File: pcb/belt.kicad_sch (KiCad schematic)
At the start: 10 parts, among them SW1 RESET, U1 Raspberry-Pi-Pico

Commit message: modified footprints
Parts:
- D1, D2: footprint (none) -> LED_THT:LED_D5.0mm
- H1, H2, H3, H4: footprint (none) -> MountingHole:MountingHole_2.7mm_M2.5
- R1, R2: footprint (none) -> Resistor_THT:R_Axial_DIN0207_L6.3mm_D2.5mm_P10.16mm_Horizontal
- SW1: footprint (none) -> Button_Switch_THT:SW_PUSH_6mm_H5mm
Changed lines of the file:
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@@
       (effects (font (size 1.27 1.27)) (justify left))
     )
-    (property "Footprint" "" (at 253.492 81.28 90)
+    (property "Footprint" "Resistor_THT:R_Axial_DIN0207_L6.3mm_D2.5mm_P10.16mm_Horizontal" (at 253.492 81.28 90)
       (effects (font (size 1.27 1.27)) hide)
     )
@@
       (effects (font (size 1.27 1.27)) (justify left))
     )
-    (property "Footprint" "" (at 234.95 114.3 0)
+    (property "Footprint" "MountingHole:MountingHole_2.7mm_M2.5" (at 234.95 114.3 0)
       (effects (font (size 1.27 1.27)) hide)
     )
@@
       (effects (font (size 1.27 1.27)) (justify right))
     )
-    (property "Footprint" "" (at 255.27 71.12 0)
+    (property "Footprint" "LED_THT:LED_D5.0mm" (at 255.27 71.12 0)
       (effects (font (size 1.27 1.27)) hide)
     )
@@
       (effects (font (size 1.27 1.27)))
     )
-    (property "Footprint" "" (at 44.45 58.42 0)
+    (property "Footprint" "Button_Switch_THT:SW_PUSH_6mm_H5mm" (at 44.45 58.42 0)
       (effects (font (size 1.27 1.27)) hide)
     )
@@
       (effects (font (size 1.27 1.27)) (justify left))
     )
-    (property "Footprint" "" (at 234.95 127 0)
+    (property "Footprint" "MountingHole:MountingHole_2.7mm_M2.5" (at 234.95 127 0)
       (effects (font (size 1.27 1.27)) hide)
     )
@@
       (effects (font (size 1.27 1.27)) (justify left))
     )
-    (property "Footprint" "" (at 234.95 133.35 0)
+    (property "Footprint" "MountingHole:MountingHole_2.7mm_M2.5" (at 234.95 133.35 0)
       (effects (font (size 1.27 1.27)) hide)
     )
@@
       (effects (font (size 1.27 1.27)) (justify left))
     )
-    (property "Footprint" "" (at 235.712 81.28 90)
+    (property "Footprint" "Resistor_THT:R_Axial_DIN0207_L6.3mm_D2.5mm_P10.16mm_Horizontal" (at 235.712 81.28 90)
       (effects (font (size 1.27 1.27)) hide)
     )
@@
       (effects (font (size 1.27 1.27)) (justify left))
     )
-    (property "Footprint" "" (at 234.95 120.65 0)
+    (property "Footprint" "MountingHole:MountingHole_2.7mm_M2.5" (at 234.95 120.65 0)
       (effects (font (size 1.27 1.27)) hide)
     )
@@
       (effects (font (size 1.27 1.27)) (justify right))
     )
-    (property "Footprint" "" (at 237.49 71.12 0)
-      (effects (font (size 1.27 1.27)) hide)
-    )
+    (property "Footprint" "LED_THT:LED_D5.0mm" (at 237.49 71.12 0)
+      (effects (font (size 1.27 1.27)) hide)
+    )

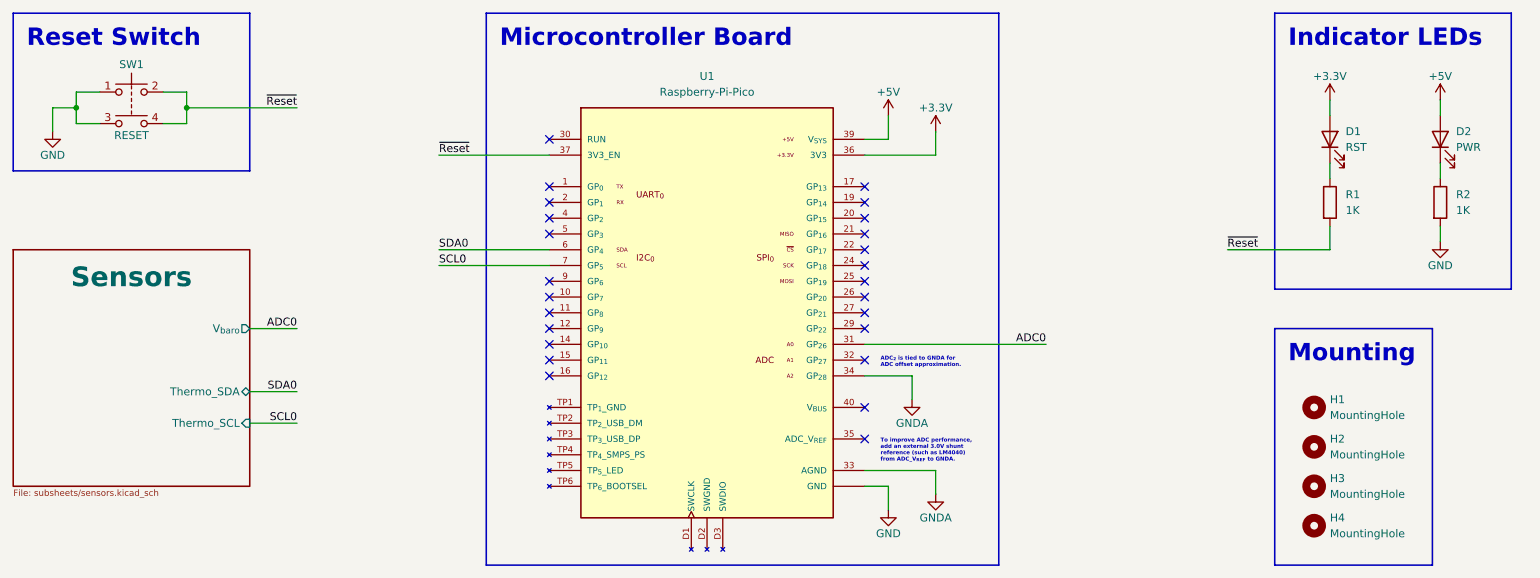
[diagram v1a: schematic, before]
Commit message: ready for layout
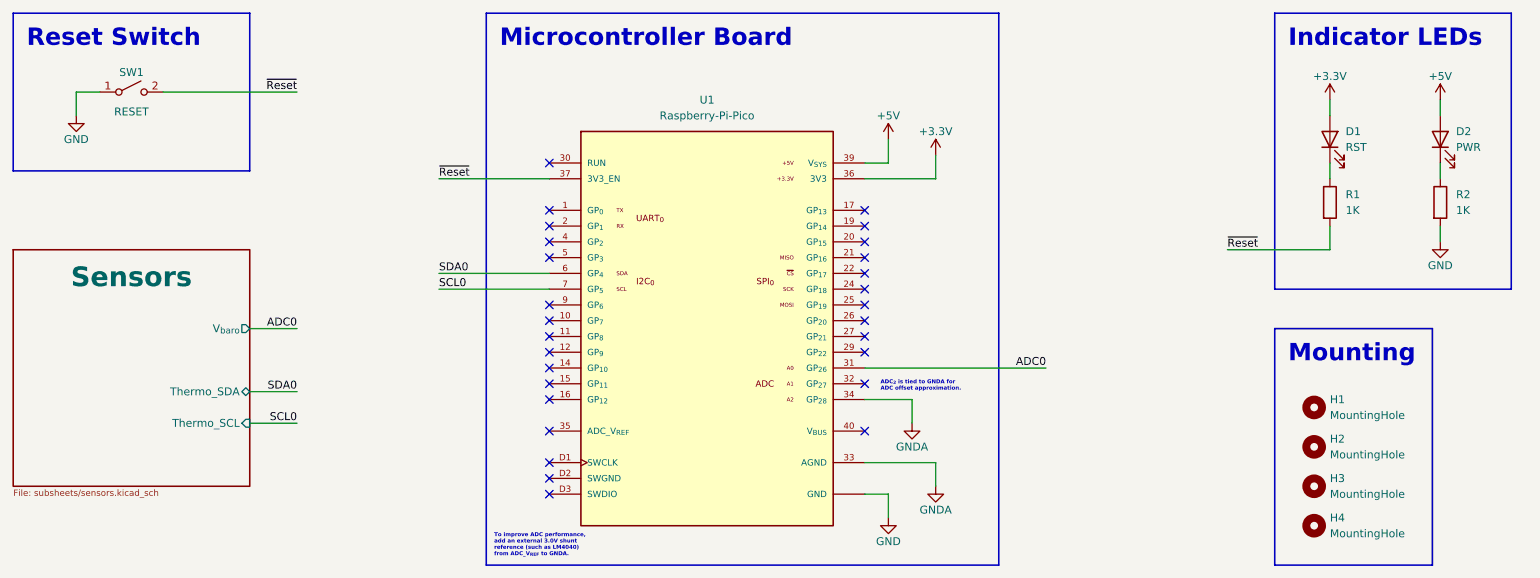
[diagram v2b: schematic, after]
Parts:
- removed SW1: RESET, Button_Switch_THT:SW_PUSH_6mm_H5mm, symbol Switch:SW_Push_Dual
- added SW1: RESET, Button_Switch_THT:SW_PUSH_6mm_H5mm, symbol Switch:SW_SPST
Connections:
- net GND: now also SW1.1 (A)
- net ~{Reset}: now also SW1.2 (B)
- no-connect marks 25 -> 28
